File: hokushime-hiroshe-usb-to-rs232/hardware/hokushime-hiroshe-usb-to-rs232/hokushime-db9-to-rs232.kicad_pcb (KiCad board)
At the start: 2 copper layers, 6 parts, among them IC1 SP3243EC/EB, U1 FT232BM/BL, U3 93CxxC

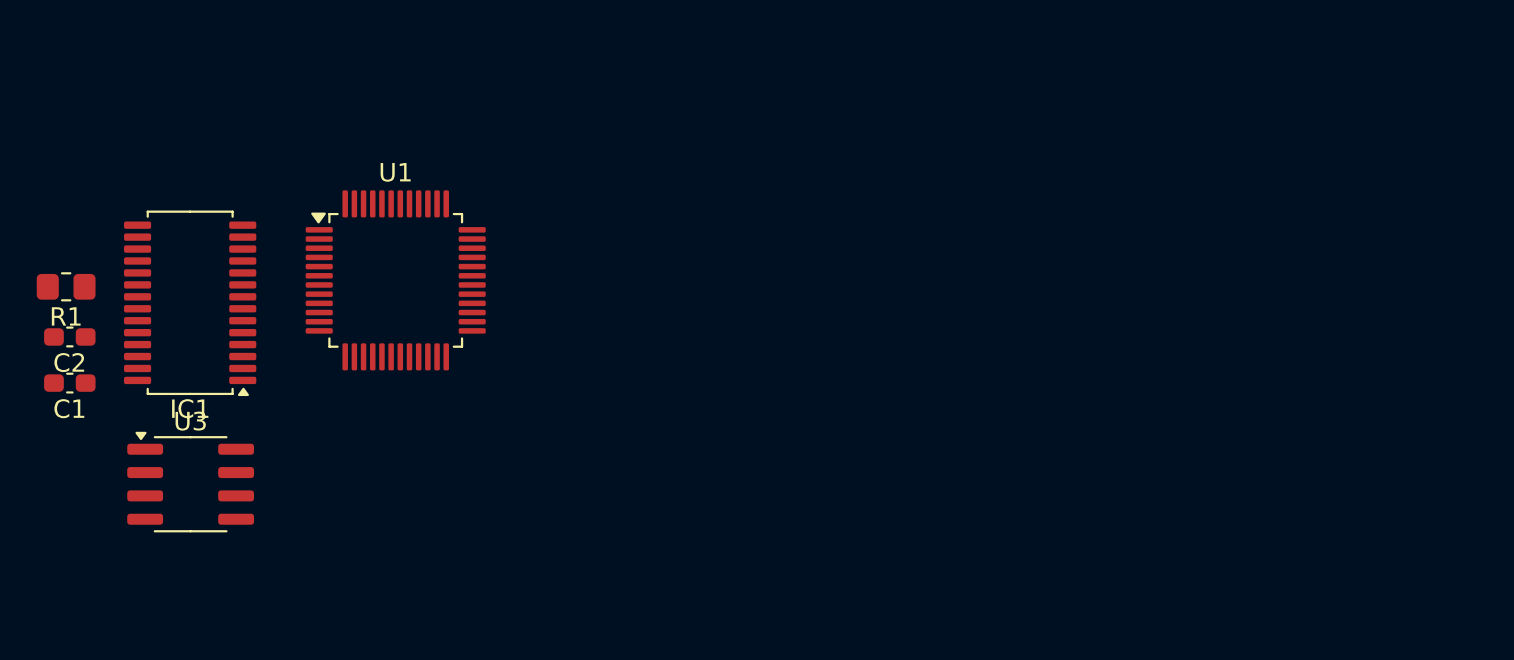
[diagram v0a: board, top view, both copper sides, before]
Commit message: [04-22-0550] Hokushime create pcb and basic layout
Update README.md
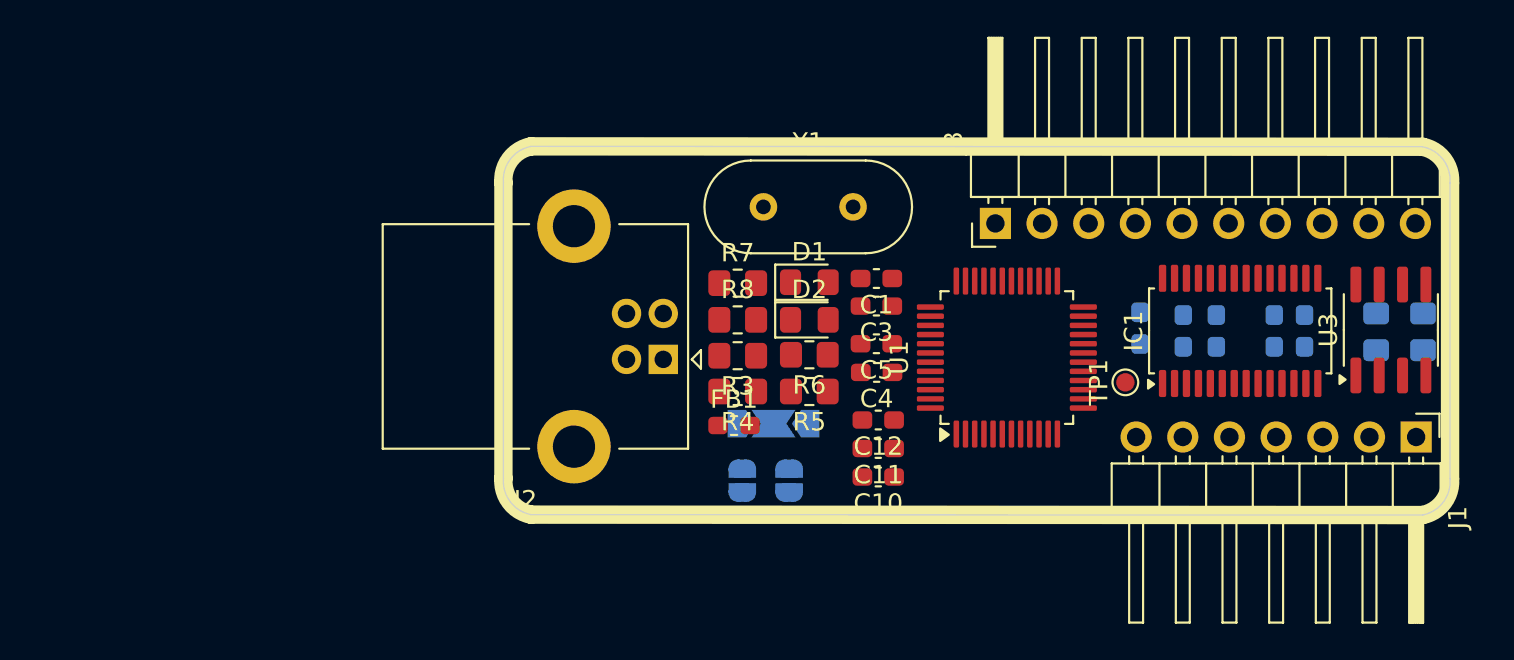
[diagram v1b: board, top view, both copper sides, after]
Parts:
- added C10: 0.1uF, Capacitor_SMD:C_0603_1608Metric_Pad1.08x0.95mm_HandSolder, F.Cu at (128.9, 98.0)
- added C11: 10uF, Capacitor_SMD:C_0603_1608Metric_Pad1.08x0.95mm_HandSolder, F.Cu at (128.9, 96.4)
- added C12: 0.1uF, Capacitor_SMD:C_0603_1608Metric_Pad1.08x0.95mm_HandSolder, F.Cu at (128.9, 94.8)
- added C3: 27pF, Capacitor_SMD:C_0603_1608Metric_Pad1.08x0.95mm_HandSolder, F.Cu at (128.8, 88.7)
- added C4: 0.1uF, Capacitor_SMD:C_0603_1608Metric_Pad1.08x0.95mm_HandSolder, F.Cu at (128.8, 92.3)
- added C5: 33nF, Capacitor_SMD:C_0603_1608Metric_Pad1.08x0.95mm_HandSolder, F.Cu at (128.8, 90.7)
- added C6: 0.22uF/16V, Capacitor_SMD:C_0603_1608Metric_Pad1.08x0.95mm_HandSolder, B.Cu at (150.4, 90.0)
- added C7: 0.22uF/16V, Capacitor_SMD:C_0603_1608Metric_Pad1.08x0.95mm_HandSolder, B.Cu at (143.2, 89.8)
- added C8: 0.22uF/16V, Capacitor_SMD:C_0603_1608Metric_Pad1.08x0.95mm_HandSolder, B.Cu at (147.3, 90.0)
- added C9: 0.22uF/16V, Capacitor_SMD:C_0603_1608Metric_Pad1.08x0.95mm_HandSolder, B.Cu at (145.5, 90.0)
- added D1: TX, LED_SMD:LED_0805_2012Metric_Pad1.15x1.40mm_HandSolder, F.Cu at (125.2, 87.3)
- added D2: RX, LED_SMD:LED_0805_2012Metric_Pad1.15x1.40mm_HandSolder, F.Cu at (125.2, 89.4)
- added FB1: 40 Ohms @100 MHz, Inductor_SMD:L_0603_1608Metric_Pad1.05x0.95mm_HandSolder, F.Cu at (121.0, 95.2)
- added G1: LOGO, external-lib:Crumbs-Logo_Footprint_13x13, B.Cu at (137.9, 94.0)
- added J1: Conn1, Connector_PinHeader_2.54mm:PinHeader_1x07_P2.54mm_Horizontal, F.Cu at (158.2, 95.8)
- added J2: USB_B, Connector_USB:USB_B_Lumberg_2411_02_Horizontal, F.Cu at (117.2, 91.5)
- added J3: Conn2, Connector_PinHeader_2.54mm:PinHeader_1x10_P2.54mm_Horizontal, F.Cu at (135.3, 84.2)
- added JP1: 5V-1, Test-2, GND-3, Jumper:SolderJumper-3_P2.0mm_Open_TrianglePad1.0x1.5mm_NumberLabels, B.Cu at (123.2, 95.0)
- added JP2: CONN2_TO_GND, Jumper:SolderJumper-2_P1.3mm_Open_RoundedPad1.0x1.5mm, B.Cu at (121.5, 98.2)
- added JP3: CONN1_SHIELD_TO_GND, Jumper:SolderJumper-2_P1.3mm_Open_RoundedPad1.0x1.5mm, B.Cu at (124.0, 98.2)
- added R2: 2K2, Resistor_SMD:R_0805_2012Metric_Pad1.20x1.40mm_HandSolder, B.Cu at (156.0, 90.0)
- added R3: 27, Resistor_SMD:R_0805_2012Metric_Pad1.20x1.40mm_HandSolder, F.Cu at (121.2, 91.3)
- added R4: 27, Resistor_SMD:R_0805_2012Metric_Pad1.20x1.40mm_HandSolder, F.Cu at (121.2, 93.3)
- added R5: 470, Resistor_SMD:R_0805_2012Metric_Pad1.20x1.40mm_HandSolder, F.Cu at (125.2, 93.3)
- added R6: 1K5, Resistor_SMD:R_0805_2012Metric_Pad1.20x1.40mm_HandSolder, F.Cu at (125.2, 91.3)
- added R7: 220, Resistor_SMD:R_0805_2012Metric_Pad1.20x1.40mm_HandSolder, F.Cu at (121.2, 87.4)
- added R8: 220, Resistor_SMD:R_0805_2012Metric_Pad1.20x1.40mm_HandSolder, F.Cu at (121.2, 89.4)
- added TP1: Status, TestPoint:TestPoint_Pad_D1.0mm, F.Cu at (142.3, 92.8)
- added Y1: 6Mhz, Crystal:Crystal_HC49-U_Vertical, F.Cu at (122.7, 83.2)
- C1: value C -> 27pF
- C2: value C_Polarized -> 0.22uF/16V; moved to B.Cu
- R1: value R_US -> 10K; moved to B.Cu
- moved R1 73.9 mm to (158.6, 90.0), turned to -90 degrees
- moved C2 67.2 mm to (152.1, 90.0), turned to 90 degrees
- moved U3 65.9 mm to (156.8, 90.0), turned to 90 degrees
- moved IC1 57.2 mm to (148.6, 90.0), turned to 90 degrees
- moved C1 44.3 mm to (128.8, 87.2)
- moved U1 33.5 mm to (135.9, 91.5), turned to 90 degrees
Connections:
- C1 pad 1: unconnected-(C1-Pad1) -> Net-(U1-XTIN)
- C1 pad 2: unconnected-(C1-Pad2) -> GND
- C2 pad 1: unconnected-(C2-Pad1) -> Net-(IC1-C1+)
- C2 pad 2: unconnected-(C2-Pad2) -> Net-(IC1-C1-)
- IC1 pad 1: unconnected-(IC1-C2+-Pad1) -> Net-(IC1-C2+)
- IC1 pad 10: unconnected-(IC1-T2OUT-Pad10) -> /CONN2_RTS
- IC1 pad 11: unconnected-(IC1-T3OUT-Pad11) -> /CONN2_DTR
- IC1 pad 12: unconnected-(IC1-T3IN-Pad12) -> /~{DTR}
- IC1 pad 13: unconnected-(IC1-T2IN-Pad13) -> /~{RTS}
- IC1 pad 14: unconnected-(IC1-T1IN-Pad14) -> /TXD
- IC1 pad 15: unconnected-(IC1-R5OUT-Pad15) -> /~{RI}
- IC1 pad 16: unconnected-(IC1-R4OUT-Pad16) -> /~{DCD}
- IC1 pad 17: unconnected-(IC1-R3OUT-Pad17) -> /~{DSR}
- IC1 pad 18: unconnected-(IC1-R2OUT-Pad18) -> /~{CTS}
- IC1 pad 19: unconnected-(IC1-R1OUT-Pad19) -> /RXD
- IC1 pad 2: unconnected-(IC1-C2--Pad2) -> Net-(IC1-C2-)
- IC1 pad 21: unconnected-(IC1-~{STATUS}-Pad21) -> Net-(IC1-~{STATUS})
- IC1 pad 22: unconnected-(IC1-~{SHUTDOWN}-Pad22) -> /~{SLEEP}
- IC1 pad 23: unconnected-(IC1-~{ONLINE}-Pad23) -> GND
- IC1 pad 24: unconnected-(IC1-C1--Pad24) -> Net-(IC1-C1-)
- IC1 pad 25: unconnected-(IC1-GND-Pad25) -> GND
- IC1 pad 26: unconnected-(IC1-VCC-Pad26) -> +5V
- IC1 pad 27: unconnected-(IC1-V+-Pad27) -> Net-(IC1-V+)
- IC1 pad 28: unconnected-(IC1-C1+-Pad28) -> Net-(IC1-C1+)
- IC1 pad 3: unconnected-(IC1-V--Pad3) -> Net-(IC1-V-)
- IC1 pad 4: unconnected-(IC1-R1IN-Pad4) -> /CONN2_RXD
- IC1 pad 5: unconnected-(IC1-R2IN-Pad5) -> /CONN2_CTS
- IC1 pad 6: unconnected-(IC1-R3IN-Pad6) -> /CONN2_DSR
- IC1 pad 7: unconnected-(IC1-R4IN-Pad7) -> /CONN2_DCD
- IC1 pad 8: unconnected-(IC1-R5IN-Pad8) -> /CONN2_RI
- IC1 pad 9: unconnected-(IC1-T1OUT-Pad9) -> /CONN2_TXD
- R1 pad 1: unconnected-(R1-Pad1) -> +5V
- R1 pad 2: unconnected-(R1-Pad2) -> /93C66_DO
- U1 pad 1: unconnected-(U1-EESK-Pad1) -> /93C66_SCLK
- U1 pad 10: unconnected-(U1-~{SLEEP}-Pad10) -> /~{SLEEP}
- U1 pad 11: unconnected-(U1-~{RXLED}-Pad11) -> Net-(U1-~{RXLED})
- U1 pad 12: unconnected-(U1-~{TXLED}-Pad12) -> Net-(U1-~{TXLED})
- U1 pad 13: unconnected-(U1-VCCIO-Pad13) -> +5V
- U1 pad 14: unconnected-(U1-PWRCTL-Pad14) -> GND
- U1 pad 17: unconnected-(U1-GND-Pad17) -> GND
- U1 pad 18: unconnected-(U1-D7/~{RI}-Pad18) -> /~{RI}
- U1 pad 19: unconnected-(U1-D6/~{DCD}-Pad19) -> /~{DCD}
- U1 pad 2: unconnected-(U1-EEDATA-Pad2) -> /93C66_DI
- U1 pad 20: unconnected-(U1-D5/~{DSR}-Pad20) -> /~{DSR}
- U1 pad 21: unconnected-(U1-D4/~{DTR}-Pad21) -> /~{DTR}
- U1 pad 22: unconnected-(U1-D3/~{CTS}-Pad22) -> /~{CTS}
- U1 pad 23: unconnected-(U1-D2/~{RST}-Pad23) -> /~{RTS}
- U1 pad 24: unconnected-(U1-D1/RXD-Pad24) -> /RXD
- U1 pad 25: unconnected-(U1-D0/TXD-Pad25) -> /TXD
- U1 pad 26: unconnected-(U1-VCC-Pad26) -> +5V
- U1 pad 27: unconnected-(U1-XTIN-Pad27) -> Net-(U1-XTIN)
- U1 pad 28: unconnected-(U1-XTOUT-Pad28) -> Net-(U1-XTOUT)
- U1 pad 29: unconnected-(U1-AGND-Pad29) -> GND
- U1 pad 3: unconnected-(U1-VCC-Pad3) -> +5V
- U1 pad 30: unconnected-(U1-AVCC-Pad30) -> Net-(U1-AVCC)
- U1 pad 31: unconnected-(U1-TEST-Pad31) -> Net-(JP1-C)
- U1 pad 32: unconnected-(U1-EECS-Pad32) -> /93C66_CS
- U1 pad 4: unconnected-(U1-~{RESET}-Pad4) -> +5V
- U1 pad 5: unconnected-(U1-~{RSTOUT}-Pad5) -> Net-(U1-~{RSTOUT})
- U1 pad 6: unconnected-(U1-3V3OUT-Pad6) -> Net-(U1-3V3OUT)
- U1 pad 7: unconnected-(U1-USBDP-Pad7) -> Net-(U1-USBDP)
- U1 pad 8: unconnected-(U1-USBDM-Pad8) -> Net-(U1-USBDM)
- U1 pad 9: unconnected-(U1-GND-Pad9) -> GND
- U3 pad 1: unconnected-(U3-CS-Pad1) -> /93C66_CS
- U3 pad 2: unconnected-(U3-SCLK-Pad2) -> /93C66_SCLK
- U3 pad 3: unconnected-(U3-DI-Pad3) -> /93C66_DI
- U3 pad 4: unconnected-(U3-DO-Pad4) -> /93C66_DO
- U3 pad 5: unconnected-(U3-GND-Pad5) -> GND
- U3 pad 6: unconnected-(U3-ORG-Pad6) -> +5V
- U3 pad 8: unconnected-(U3-VCC-Pad8) -> +5V
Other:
- board outline added: 51.5 x 20.1 mm
- board text added: "HOKUSHIME"

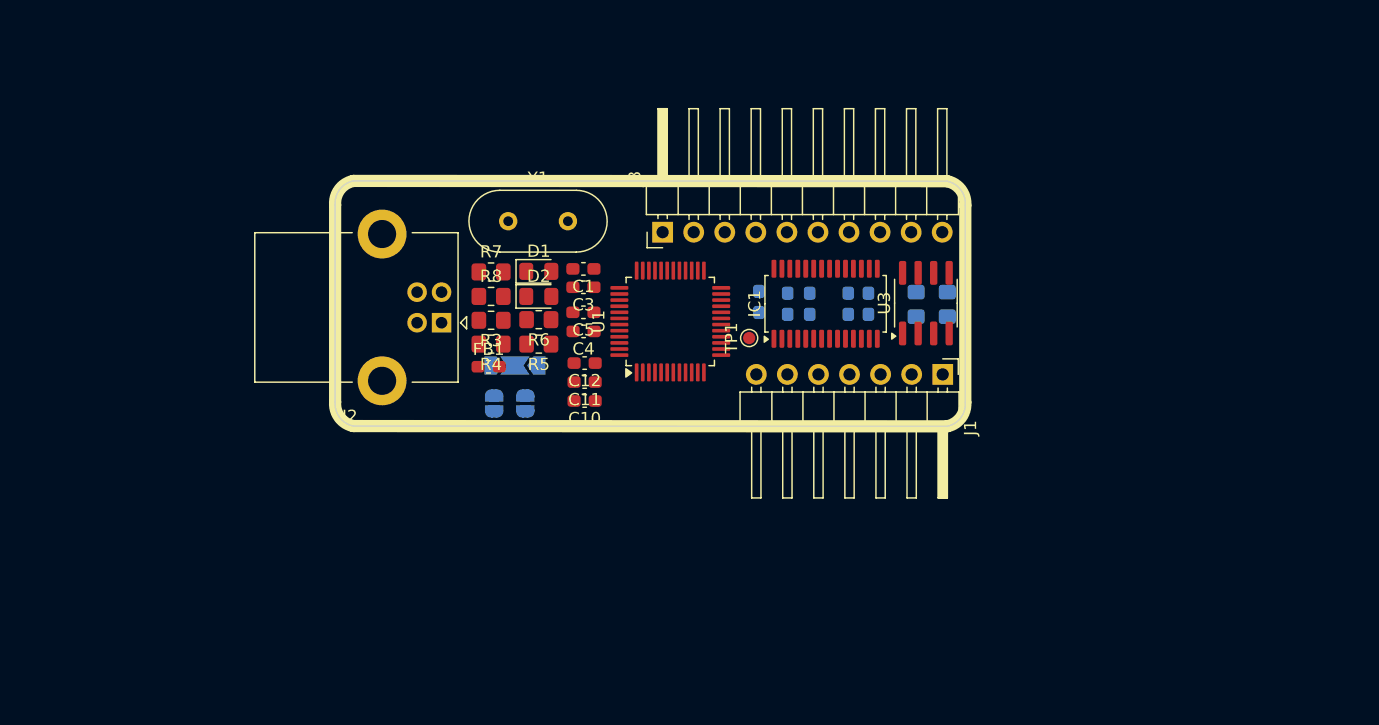
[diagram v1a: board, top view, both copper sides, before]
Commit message: [04-22-1840] thing about vias making
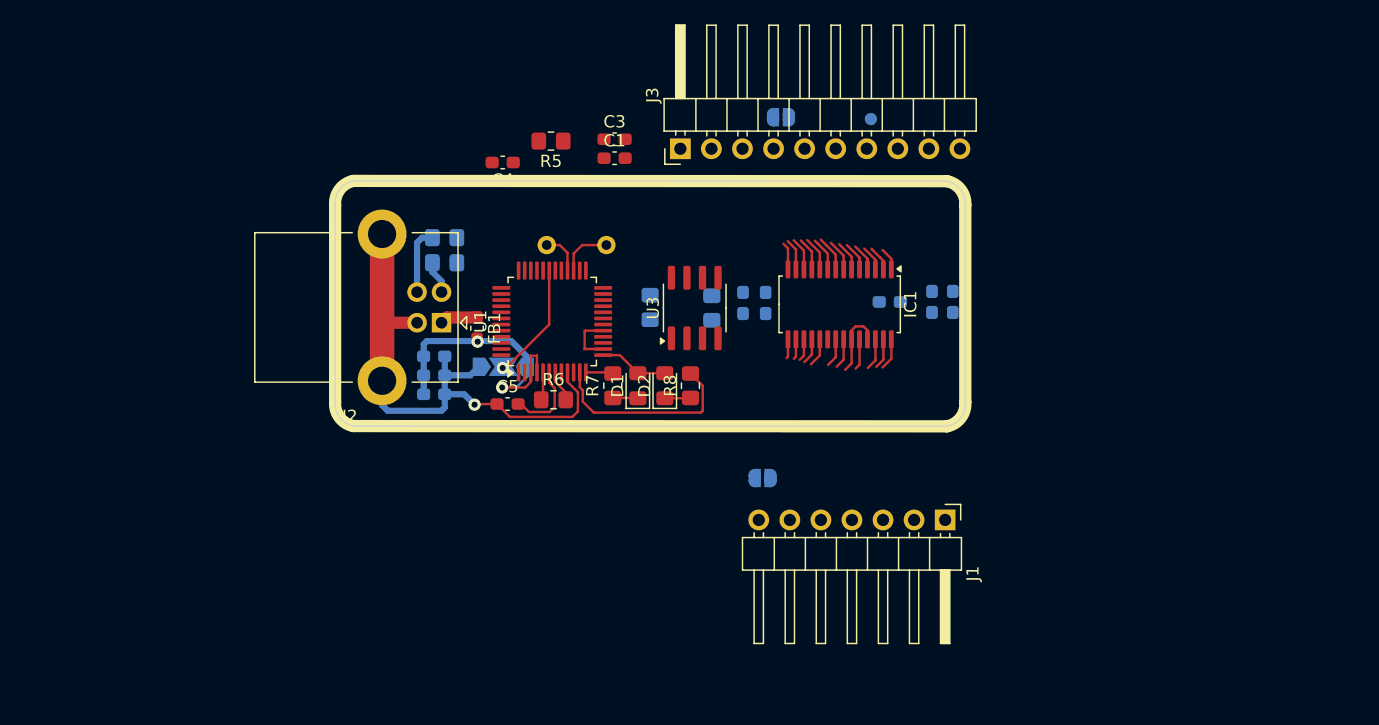
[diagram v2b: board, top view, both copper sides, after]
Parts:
- C10, C11, C12, R3, R4, TP1, Y1: moved to B.Cu
- moved JP2 33.1 mm to (144.9, 74.8), turned to 180 degrees
- moved R2 21.8 mm to (134.2, 90.3)
- moved TP1 20.5 mm to (152.3, 74.9)
- moved JP3 20.3 mm to (143.4, 104.2), turned to 180 degrees
- moved R1 19.3 mm to (139.3, 90.3)
- moved U3 18.9 mm to (137.9, 90.3)
- moved R8 17.9 mm to (137.6, 96.7), turned to 90 degrees
- moved R5 16.6 mm to (126.2, 76.7)
- moved C7 15.8 mm to (159.0, 89.8)
- moved C4 15.3 mm to (122.2, 78.5)
- moved R7 13.6 mm to (131.2, 96.7), turned to 90 degrees
- moved D2 12.6 mm to (135.4, 96.7), turned to 90 degrees
- moved D1 12.4 mm to (133.2, 96.7), turned to 90 degrees
- moved C3 12.4 mm to (131.3, 76.5), turned to 0 degrees
- moved C12 12.3 mm to (116.6, 94.3)
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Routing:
- net GND: track 0.00 -> 55.2 mm, vias 0 -> 1
- net +5V: track 0.00 -> 32.3 mm, vias 0 -> 2
- net Net-(U1-~{RXLED}): track 0.00 -> 16.2 mm
- net Net-(JP1-C): track 0.00 -> 9.80 mm, vias 0 -> 1
- net Net-(U1-3V3OUT): track 0.00 -> 6.44 mm
- net /USBD+: track 0.00 -> 5.47 mm
- net Net-(U1-XTIN): track 0.00 -> 4.36 mm
- net Net-(U1-XTOUT): track 0.00 -> 3.41 mm
- net VBUS: track 0.00 -> 3.08 mm
- net /CONN2_RI: track 0.00 -> 2.94 mm
- net /CONN2_RTS: track 0.00 -> 2.82 mm
- net /CONN2_TXD: track 0.00 -> 2.79 mm
- net /CONN2_DTR: track 0.00 -> 2.73 mm
- net /~{DTR}: track 0.00 -> 2.72 mm
- net /USBD-: track 0.00 -> 2.71 mm
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
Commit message: [04-24-1904] pcb routing finished
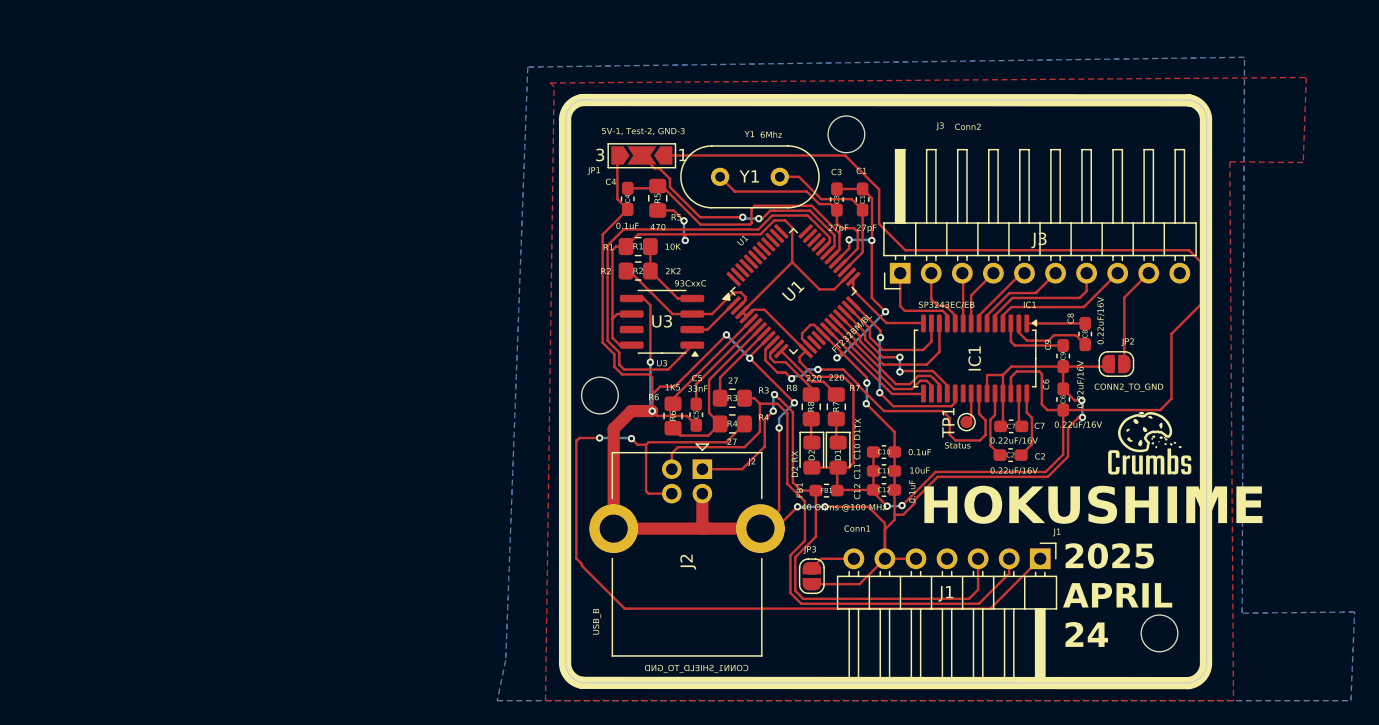
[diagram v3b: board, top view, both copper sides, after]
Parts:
- added G1: LOGO, external-lib:Crumbs-Logo_Footprint_13x13, F.Cu at (174.9, 101.2)
- added H1: MountingHole, MountingHole:MountingHole_3mm, F.Cu at (150.3, 76.2)
- added H2: MountingHole, MountingHole:MountingHole_3mm, F.Cu at (130.2, 97.5)
- added H4: MountingHole, MountingHole:MountingHole_3mm, F.Cu at (175.9, 117.0)
- C10, C11, C12, C2, C6, C7, C8, C9, JP1, JP2, JP3, R1, R2, R3, R4, TP1, Y1: moved to F.Cu
- moved C12 38.4 mm to (153.4, 105.2)
- moved C11 37.6 mm to (153.4, 103.7)
- moved C10 37.1 mm to (153.4, 102.1)
- moved G1 35.8 mm to (166.3, 115.8)
- moved JP2 34.0 mm to (172.4, 94.9)
- moved FB1 31.5 mm to (148.7, 105.3), turned to 0 degrees
- moved R4 28.0 mm to (141.0, 99.8), turned to 0 degrees
- moved R3 26.0 mm to (141.0, 97.7), turned to 0 degrees
- moved TP1 26.0 mm to (160.1, 99.7)
- moved C6 25.6 mm to (168.0, 97.8), turned to 90 degrees
- moved C2 25.2 mm to (163.7, 102.4), turned to 180 degrees
- moved J2 24.5 mm to (138.5, 103.5), turned to -90 degrees
- moved JP1 20.7 mm to (133.6, 77.9)
- moved J3 20.7 mm to (154.7, 87.5)
- moved C1 20.6 mm to (151.6, 81.5), turned to 90 degrees
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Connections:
- J3 pad 2: /CONN2_TXD -> /CONN2_RTS
- J3 pad 3: /CONN2_RXD -> /CONN2_TXD
- J3 pad 4: /CONN2_DSR -> /CONN2_RI
- J3 pad 5: /CONN2_GND -> /CONN2_DCD
- J3 pad 6: /CONN2_DCD -> /CONN2_DSR
- J3 pad 8: /CONN2_RTS -> /CONN2_RXD
- J3 pad 9: /CONN2_RI -> /CONN2_GND
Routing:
- net GND: track 55.2 -> 210.9 mm, vias 1 -> 16
- net +5V: track 32.3 -> 178.1 mm, vias 2 -> 4
- net /USBD+: track 5.47 -> 71.8 mm, vias 0 -> 2
- net /USBD-: track 2.71 -> 51.8 mm
- net VBUS: track 3.08 -> 47.4 mm, vias 0 -> 2
- net /93C66_CS: track 0.00 -> 38.2 mm
- net /~{SLEEP}: track 2.48 -> 27.7 mm, vias 0 -> 2
- net Net-(U1-AVCC): track 0.00 -> 23.2 mm
- net Net-(U1-XTOUT): track 3.41 -> 17.1 mm
- net /RXD: track 2.34 -> 15.7 mm, vias 0 -> 2
- net /93C66_DI: track 0.00 -> 13.3 mm
- net Net-(U1-USBDP): track 2.69 -> 14.3 mm
- net Net-(JP1-C): track 9.80 -> 21.1 mm, vias 1 -> 2
- net /~{CTS}: track 2.11 -> 12.6 mm, vias 0 -> 2
- net /~{DSR}: track 1.81 -> 12.1 mm
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- added copper zone on F.Cu, net +5V
- added copper zone on B.Cu, net GND
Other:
- board size 51.5 x 20.1 mm -> 52.4 x 47.7 mm
- board text added: "2025 APRIL 24"
- board text added: "Assembled with Love and a soldering iron Powered by electrons and good vibes 01010011 01101111 01101100 01100100 01100101 01110010 00100001 Debug me if you can Built with coffe and late-night commits This PCB contains 0% AI. 100% sweat. Code, solder, coffee, repeat Beep Boop Circuit Activated Open source. Open heart. Closed loops. This board was debugged with mild panic"
